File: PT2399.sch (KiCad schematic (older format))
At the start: 43 parts, among them J1 Output Jack, J2 Input Jack, J3 Jack-DC, U1 L78L05_TO92, U2 PT2399, U3 TL072

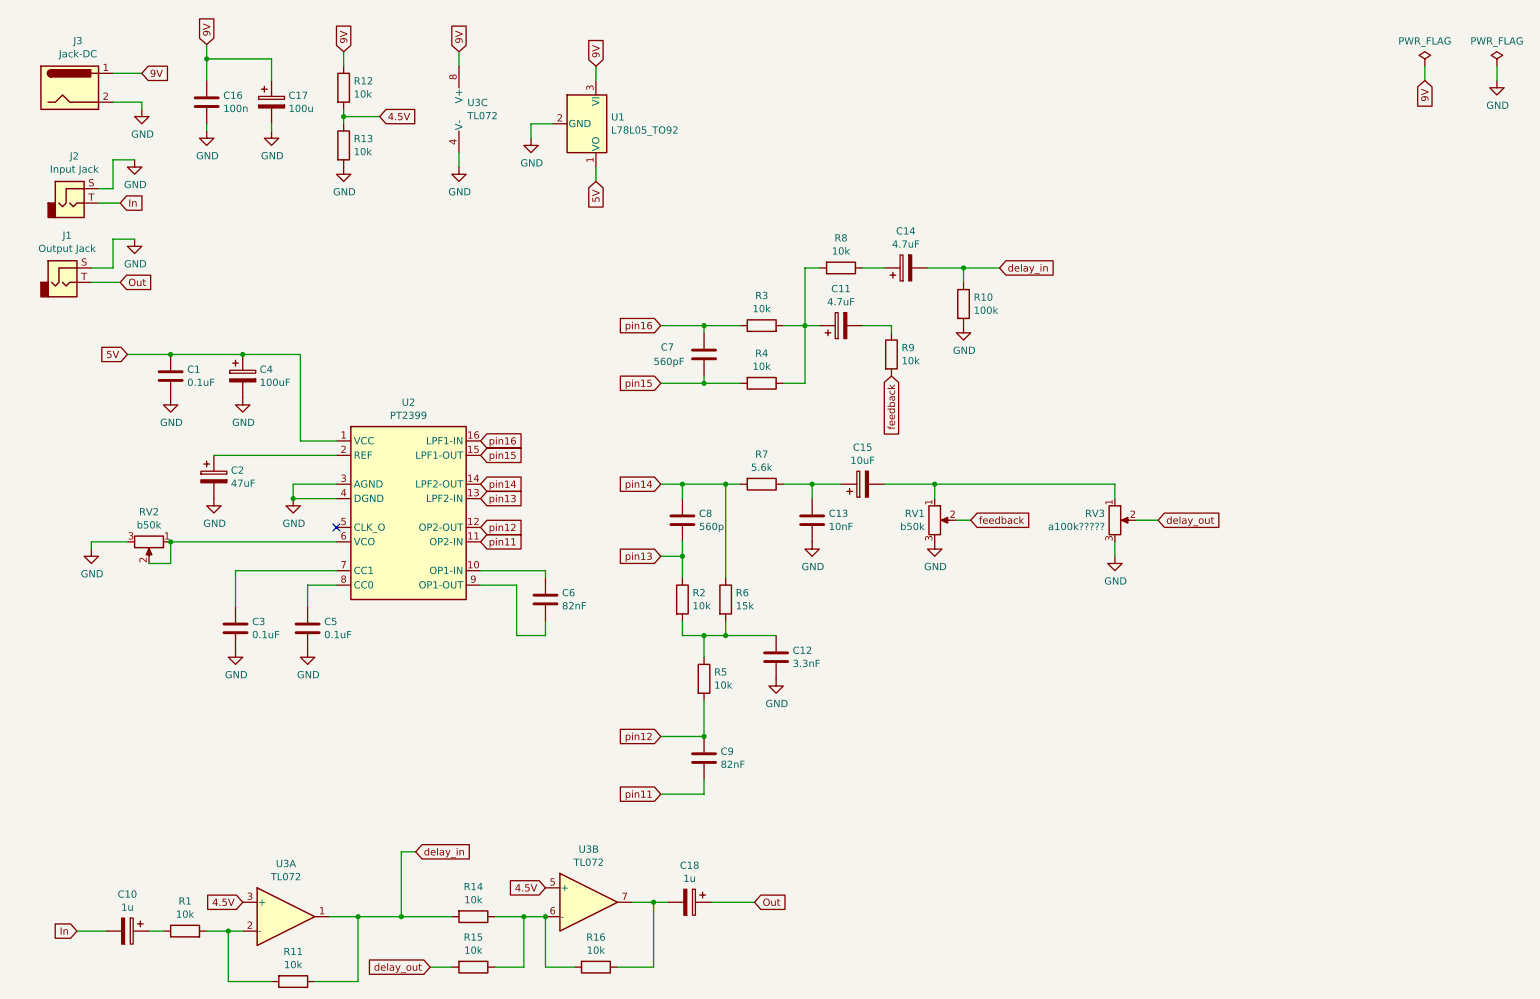
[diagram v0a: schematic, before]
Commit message: stuff
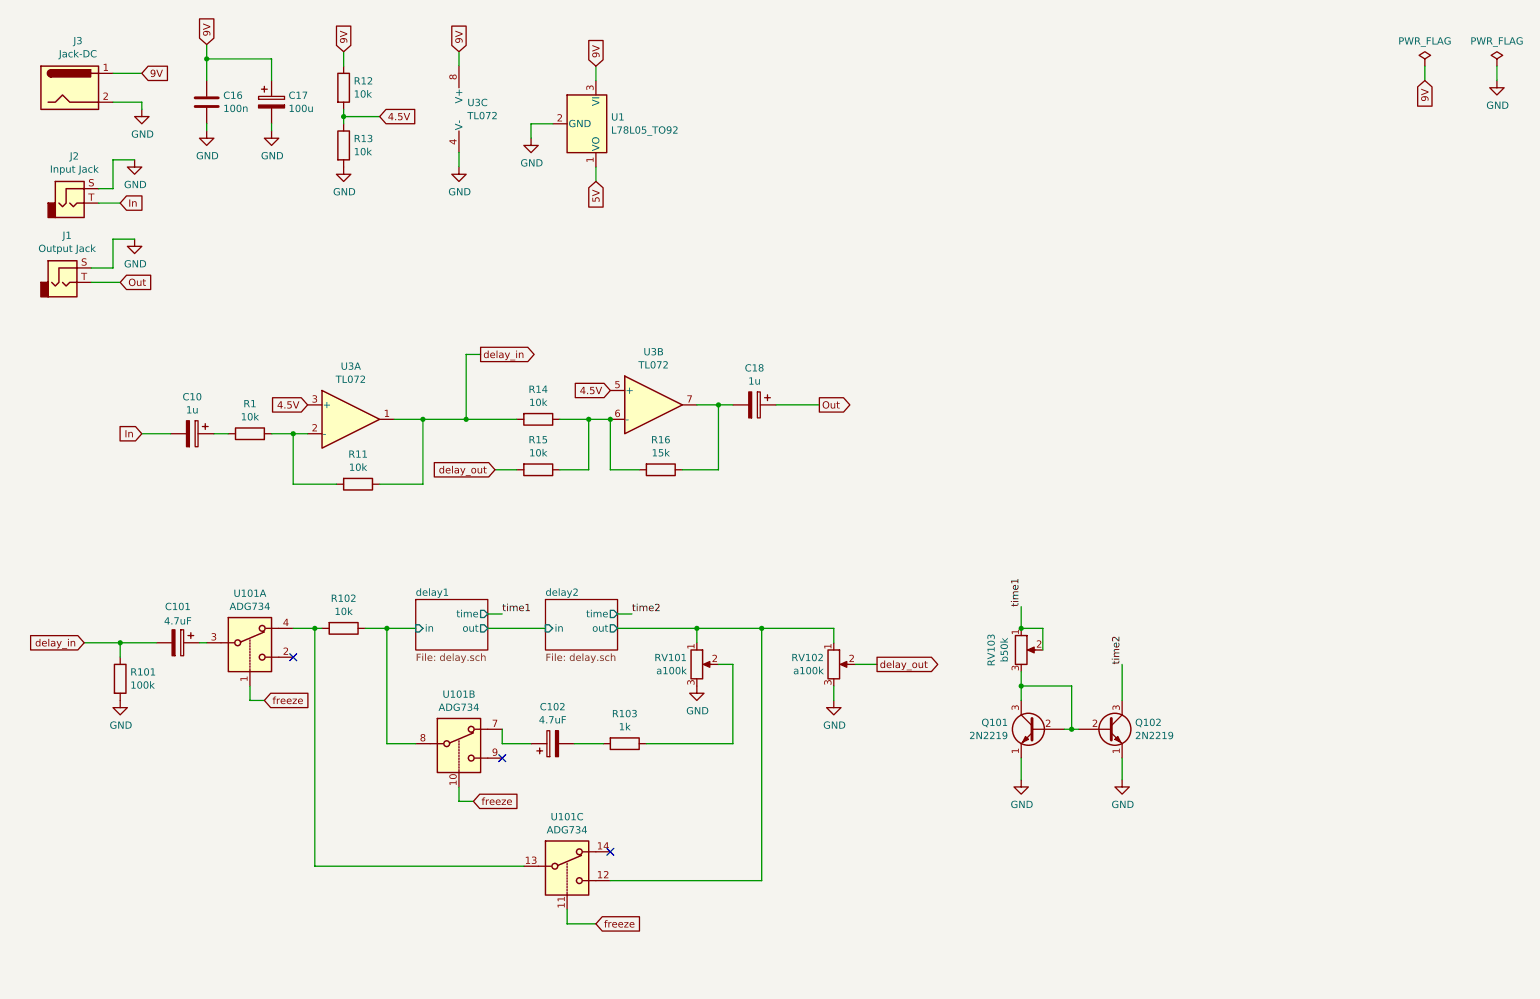
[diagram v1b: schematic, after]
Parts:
- removed C1, C3, C5: 0.1uF, symbol Device:C
- removed C11, C14: 4.7uF, symbol Device:CP
- removed C12: 3.3nF, symbol Device:C
- removed C13: 10nF, symbol Device:C
- removed C15: 10uF, symbol Device:CP
- removed C2: 47uF, symbol Device:CP
- removed C4: 100uF, symbol Device:CP
- removed C6, C9: 82nF, symbol Device:C
- removed C7: 560pF, symbol Device:C
- removed C8: 560p, symbol Device:C
- removed R10: 100k, symbol Device:R
- removed R2, R3, R4, R5, R8, R9: 10k, symbol Device:R
- removed R6: 15k, symbol Device:R
- removed R7: 5.6k, symbol Device:R
- removed RV1, RV2: b50k, symbol Device:R_POT
- removed RV3: a100k?????, symbol Device:R_POT
- removed U2: PT2399, symbol Audio:PT2399
- added C101, C102: 4.7uF, symbol Device:CP
- added Q101, Q102: 2N2219, Package_TO_SOT_THT:TO-39-3, symbol Transistor_BJT:2N2219
- added R101: 100k, symbol Device:R
- added R102: 10k, symbol Device:R
- added R103: 1k, symbol Device:R
- added RV101, RV102: a100k, symbol Device:R_POT
- added RV103: b50k, symbol Device:R_POT
- added U101: ADG734, Package_SO:TSSOP-20_4.4x6.5mm_P0.65mm, symbol Analog_Switch:ADG734
- R16: value 10k -> 15k
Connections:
- net GND: now also Q101.1 (E), Q102.1 (E), R101.2, RV101.3, RV102.3
- net delay_in: now also C101.2, R101.1
- net delay_out: now also RV102.2
- new net: R103.1, RV101.2
- new net: C102.1, U101.7
- new net: C102.2, R103.2
- new net: C101.1, U101.3
- new net: R102.2, U101.13, U101.4
- new net: Q101.2 (B), Q101.3 (C), Q102.2 (B), RV103.3
- new net delay1/in: R102.1, U101.8
- new net delay2/out: RV101.1, RV102.1, U101.12
- new net freeze: U101.1, U101.10, U101.11
- new net time1: RV103.1, RV103.2
- new net time2: Q102.3 (C)
- no-connect marks 1 -> 3
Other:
- moved on the sheet: C10, C18, R1, R11, R14, R15, R16, U3A, U3B
